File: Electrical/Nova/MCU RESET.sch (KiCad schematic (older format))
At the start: 7 parts

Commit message: And Another one....
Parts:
- removed C401, C402: 10pf, NOVA MCU (STM):C_0805_2012Metric_Pad1.15x1.40mm_HandSolder, symbol Nova_Microcontroller:C
- removed C403, C404: 18pf, NOVA MCU (STM):C_0805_2012Metric_Pad1.15x1.40mm_HandSolder, symbol Nova_Microcontroller:C
- removed R?: TBD, NOVA MCU (STM):R_0805_2012Metric_Pad1.15x1.40mm_HandSolder, symbol Nova_Microcontroller:R_US
- removed Y?: ECS-260-8-36B-CKY-TR, NOVA MCU (STM):ECX-2236B, symbol Nova_Microcontroller:Crystal_GND24
- removed Y?: JTX310, NOVA MCU (STM):JTX310, symbol Nova_Microcontroller:Crystal
- added C?: 0.1uF, NOVA MCU (STM):C_0805_2012Metric_Pad1.15x1.40mm_HandSolder, symbol Nova_Microcontroller:C
- added S?: KSR223GLFG, NOVA MCU (STM):KSR223GLFG, symbol Nova_Microcontroller:GPTS203211B
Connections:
- net labels added: RESET
- net labels removed: CLOCKIN, CLOCKOUT, RTCCRYSTALIN, RTCCRYSTALOUT
- wire segments 12 -> 3

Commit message: Added Barometer, Flash, SD, and Power Supply
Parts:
- C?: symbol Nova_Microcontroller:C -> Nova-rescue:C-Nova_Microcontroller
- S?: symbol Nova_Microcontroller:GPTS203211B -> Nova-rescue:GPTS203211B-Nova_Microcontroller
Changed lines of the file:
@@
 $Descr A4 11693 8268
 encoding utf-8
-Sheet 8 9
+Sheet 8 13
 Title "Microcontroller"
 Date "2020-07-02"
@@
 $EndBitmap
 $Comp
-L Nova_Microcontroller:GPTS203211B S?
+L Nova-rescue:GPTS203211B-Nova_Microcontroller S?
 U 1 1 5EEE3482
 P 5700 3550
@@
 RESET
 $Comp
-L Nova_Microcontroller:C C?
+L Nova-rescue:C-Nova_Microcontroller C?
 U 1 1 5EEE5880
 P 6350 3700

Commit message: Fixed Power Supply
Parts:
- C?: symbol Nova-rescue:C-Nova_Microcontroller -> Nova-rescue:C-Nova_Microcontroller-Nova-rescue
- S?: symbol Nova-rescue:GPTS203211B-Nova_Microcontroller -> Nova-rescue:GPTS203211B-Nova_Microcontroller-Nova-rescue
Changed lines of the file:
@@
 $EndBitmap
 $Comp
-L Nova-rescue:GPTS203211B-Nova_Microcontroller S?
+L Nova-rescue:GPTS203211B-Nova_Microcontroller-Nova-rescue S?
 U 1 1 5EEE3482
 P 5700 3550
@@
 RESET
 $Comp
-L Nova-rescue:C-Nova_Microcontroller C?
+L Nova-rescue:C-Nova_Microcontroller-Nova-rescue C?
 U 1 1 5EEE5880
 P 6350 3700

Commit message: Added Gyroscope
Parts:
- C?: symbol Nova-rescue:C-Nova_Microcontroller-Nova-rescue -> Nova-rescue:C-Nova_Microcontroller-Nova-rescue-Nova-rescue
- S?: symbol Nova-rescue:GPTS203211B-Nova_Microcontroller-Nova-rescue -> Nova-rescue:GPTS203211B-Nova_Microcontroller-Nova-rescue-Nova-rescue
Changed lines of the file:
@@
 $Descr A4 11693 8268
 encoding utf-8
-Sheet 8 13
+Sheet 8 14
 Title "Microcontroller"
 Date "2020-07-02"
@@
 $EndBitmap
 $Comp
-L Nova-rescue:GPTS203211B-Nova_Microcontroller-Nova-rescue S?
+L Nova-rescue:GPTS203211B-Nova_Microcontroller-Nova-rescue-Nova-rescue S?
 U 1 1 5EEE3482
 P 5700 3550
@@
 RESET
 $Comp
-L Nova-rescue:C-Nova_Microcontroller-Nova-rescue C?
+L Nova-rescue:C-Nova_Microcontroller-Nova-rescue-Nova-rescue C?
 U 1 1 5EEE5880
 P 6350 3700

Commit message: Added Gyro pins. Organized Schematic
Need to determine if we need the interrupt pins for the sensors.
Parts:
- C?: symbol Nova-rescue:C-Nova_Microcontroller-Nova-rescue-Nova-rescue -> Nova-rescue:C-Nova_Microcontroller-Nova-rescue-Nova-rescue-Nova-rescue
- S?: symbol Nova-rescue:GPTS203211B-Nova_Microcontroller-Nova-rescue-Nova-rescue -> Nova-rescue:GPTS203211B-Nova_Microcontroller-Nova-rescue-Nova-rescue-Nova-rescue
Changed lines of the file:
@@
 $EndBitmap
 $Comp
-L Nova-rescue:GPTS203211B-Nova_Microcontroller-Nova-rescue-Nova-rescue S?
+L Nova-rescue:GPTS203211B-Nova_Microcontroller-Nova-rescue-Nova-rescue-Nova-rescue S?
 U 1 1 5EEE3482
 P 5700 3550
@@
 RESET
 $Comp
-L Nova-rescue:C-Nova_Microcontroller-Nova-rescue-Nova-rescue C?
+L Nova-rescue:C-Nova_Microcontroller-Nova-rescue-Nova-rescue-Nova-rescue C?
 U 1 1 5EEE5880
 P 6350 3700

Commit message: Added Pyro Channels
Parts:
- C?: symbol Nova-rescue:C-Nova_Microcontroller-Nova-rescue-Nova-rescue-Nova-rescue -> Nova-rescue:C-Nova_Microcontroller-Nova-rescue-Nova-rescue-Nova-rescue-Nova-rescue
- S?: symbol Nova-rescue:GPTS203211B-Nova_Microcontroller-Nova-rescue-Nova-rescue-Nova-rescue -> Nova-rescue:GPTS203211B-Nova_Microcontroller-Nova-rescue-Nova-rescue-Nova-rescue-Nova-rescue
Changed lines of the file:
@@
 $Descr A4 11693 8268
 encoding utf-8
-Sheet 8 14
+Sheet 8 16
 Title "Microcontroller"
 Date "2020-07-02"
@@
 $EndBitmap
 $Comp
-L Nova-rescue:GPTS203211B-Nova_Microcontroller-Nova-rescue-Nova-rescue-Nova-rescue S?
+L Nova-rescue:GPTS203211B-Nova_Microcontroller-Nova-rescue-Nova-rescue-Nova-rescue-Nova-rescue S?
 U 1 1 5EEE3482
 P 5700 3550
@@
 RESET
 $Comp
-L Nova-rescue:C-Nova_Microcontroller-Nova-rescue-Nova-rescue-Nova-rescue C?
+L Nova-rescue:C-Nova_Microcontroller-Nova-rescue-Nova-rescue-Nova-rescue-Nova-rescue C?
 U 1 1 5EEE5880
 P 6350 3700

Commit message: Added LED sheet and pins
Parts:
- C?: symbol Nova-rescue:C-Nova_Microcontroller-Nova-rescue-Nova-rescue-Nova-rescue-Nova-rescue -> Nova-rescue:C-Nova_Microcontroller-Nova-rescue-Nova-rescue-Nova-rescue-Nova-rescue-Nova-rescue
- S?: symbol Nova-rescue:GPTS203211B-Nova_Microcontroller-Nova-rescue-Nova-rescue-Nova-rescue-Nova-rescue -> Nova-rescue:GPTS203211B-Nova_Microcontroller-Nova-rescue-Nova-rescue-Nova-rescue-Nova-rescue-Nova-rescue
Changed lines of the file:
@@
 $Descr A4 11693 8268
 encoding utf-8
-Sheet 8 16
+Sheet 8 18
 Title "Microcontroller"
 Date "2020-07-02"
@@
 $EndBitmap
 $Comp
-L Nova-rescue:GPTS203211B-Nova_Microcontroller-Nova-rescue-Nova-rescue-Nova-rescue-Nova-rescue S?
+L Nova-rescue:GPTS203211B-Nova_Microcontroller-Nova-rescue-Nova-rescue-Nova-rescue-Nova-rescue-Nova-rescue S?
 U 1 1 5EEE3482
 P 5700 3550
@@
 RESET
 $Comp
-L Nova-rescue:C-Nova_Microcontroller-Nova-rescue-Nova-rescue-Nova-rescue-Nova-rescue C?
+L Nova-rescue:C-Nova_Microcontroller-Nova-rescue-Nova-rescue-Nova-rescue-Nova-rescue-Nova-rescue C?
 U 1 1 5EEE5880
 P 6350 3700

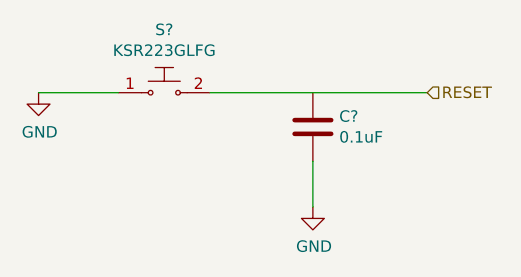
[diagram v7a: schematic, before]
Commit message: Minor update
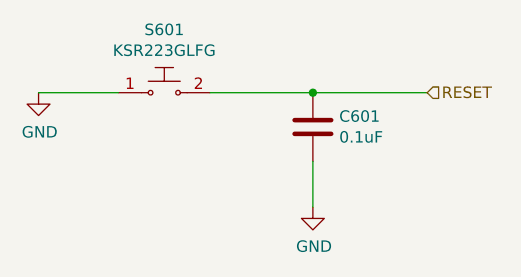
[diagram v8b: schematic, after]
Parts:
- C601: renamed from C?; footprint NOVA MCU (STM):C_0805_2012Metric_Pad1.15x1.40mm_HandSolder -> NOVA MCU (STM):C_0805_2012Metric
- gave numbers to parts that had none: 1
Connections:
- net RESET: now also C601.1
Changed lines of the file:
@@
 $Descr A4 11693 8268
 encoding utf-8
-Sheet 8 18
+Sheet 6 18
 Title "Microcontroller"
 Date "2020-07-02"
@@
 $EndBitmap
 $Comp
-L Nova-rescue:GPTS203211B-Nova_Microcontroller-Nova-rescue-Nova-rescue-Nova-rescue-Nova-rescue-Nova-rescue S?
+L Nova-rescue:GPTS203211B-Nova_Microcontroller-Nova-rescue-Nova-rescue-Nova-rescue-Nova-rescue-Nova-rescue S601
 U 1 1 5EEE3482
 P 5700 3550
-F 0 "S?" H 5700 3825 50  0000 C CNN
+F 0 "S601" H 5700 3825 50  0000 C CNN
 F 1 "KSR223GLFG" H 5700 3734 50  0000 C CNN
 F 2 "NOVA MCU (STM):KSR223GLFG" H 5900 3750 50  0001 L CNN
@@
 $EndComp
 $Comp
-L power:GND #PWR?
+L power:GND #PWR0601
 U 1 1 5EEE4440
 P 5150 3550
-F 0 "#PWR?" H 5150 3300 50  0001 C CNN
+F 0 "#PWR0601" H 5150 3300 50  0001 C CNN
 F 1 "GND" H 5155 3377 50  0000 C CNN
 F 2 "" H 5150 3550 50  0001 C CNN
@@
 	5150 3550 5500 3550
 $Comp
-L power:GND #PWR?
+L power:GND #PWR0602
 U 1 1 5EEE4D7F
 P 6350 4050
-F 0 "#PWR?" H 6350 3800 50  0001 C CNN
+F 0 "#PWR0602" H 6350 3800 50  0001 C CNN
 F 1 "GND" H 6355 3877 50  0000 C CNN
 F 2 "" H 6350 4050 50  0001 C CNN
@@
 RESET
 $Comp
-L Nova-rescue:C-Nova_Microcontroller-Nova-rescue-Nova-rescue-Nova-rescue-Nova-rescue-Nova-rescue C?
+L Nova-rescue:C-Nova_Microcontroller-Nova-rescue-Nova-rescue-Nova-rescue-Nova-rescue-Nova-rescue C601
 U 1 1 5EEE5880
 P 6350 3700
-F 0 "C?" H 6465 3746 50  0000 L CNN
+F 0 "C601" H 6465 3746 50  0000 L CNN
 F 1 "0.1uF" H 6465 3655 50  0000 L CNN
-F 2 "NOVA MCU (STM):C_0805_2012Metric_Pad1.15x1.40mm_HandSolder" H 6388 3550 50  0001 C CNN
+F 2 "NOVA MCU (STM):C_0805_2012Metric" H 6388 3550 50  0001 C CNN
 F 3 "~" H 6350 3700 50  0001 C CNN
 	1    6350 3700
@@
 $EndBitmap
 Wire Wire Line
-	5900 3550 6850 3550
+	5900 3550 6350 3550
+Connection ~ 6350 3550
+Wire Wire Line
+	6350 3550 6850 3550
 $EndSCHEMATC
